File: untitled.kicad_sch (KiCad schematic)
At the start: 18 parts, among them J4 Pyro 2, J5 Pyro 1, Q1 FDS9926A, Q2 FDS4953, Q3 NDT3055L

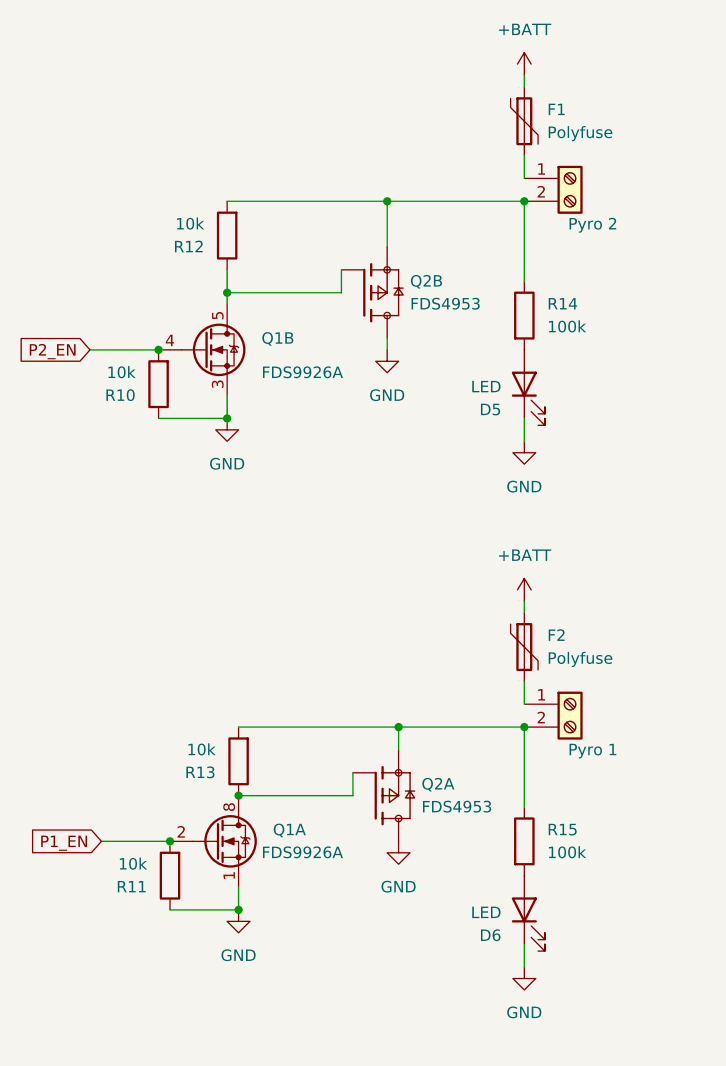
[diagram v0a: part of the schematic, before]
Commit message: V3
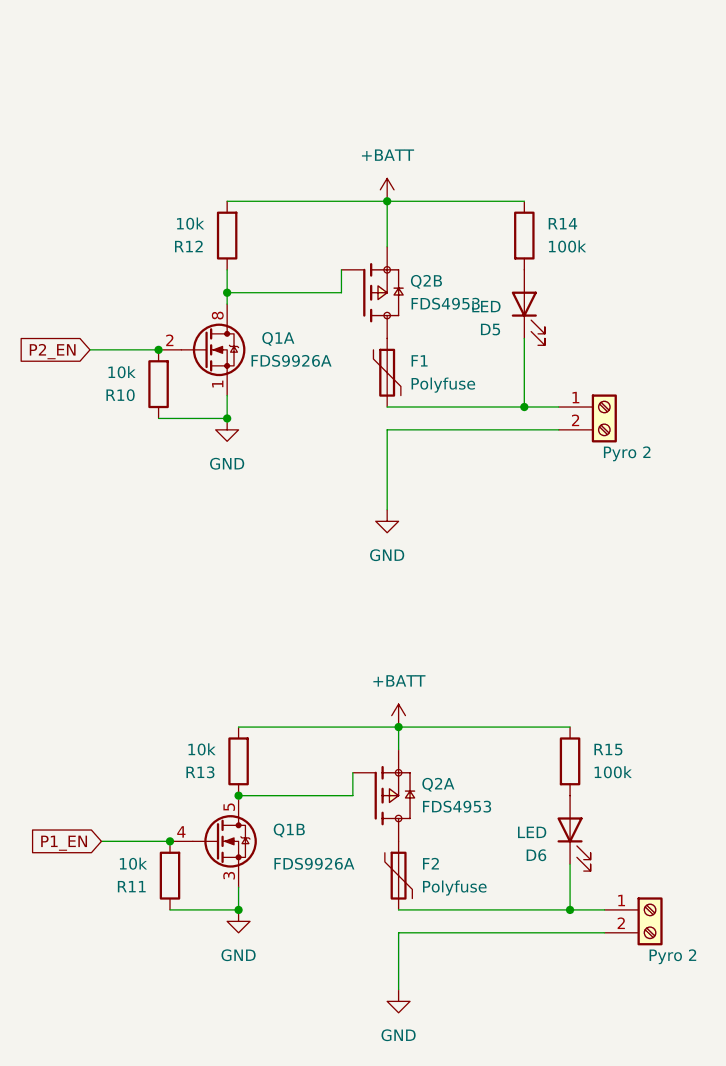
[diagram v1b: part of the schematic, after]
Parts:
- J4: footprint TerminalBlock_4Ucon:TerminalBlock_4Ucon_1x02_P3.50mm_Vertical -> TerminalBlock_Phoenix:TerminalBlock_Phoenix_MPT-0,5-2-2.54_1x02_P2.54mm_Horizontal
- J5: value Pyro 1 -> Pyro 2; footprint TerminalBlock_4Ucon:TerminalBlock_4Ucon_1x02_P3.50mm_Vertical -> TerminalBlock_Phoenix:TerminalBlock_Phoenix_MPT-0,5-2-2.54_1x02_P2.54mm_Horizontal
- Q3: footprint Package_TO_SOT_SMD:TSOT-23_HandSoldering -> Package_TO_SOT_SMD:TSOT-23
- R10, R11, R12, R13, R14, R15, R17, R18: footprint Resistor_SMD:R_0603_1608Metric_Pad0.98x0.95mm_HandSolder -> Resistor_SMD:R_0402_1005Metric_Pad0.72x0.64mm_HandSolder
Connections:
- net +BATT: now also Q2.1, Q2.3, R12.2, R13.2, R14.1, R15.1; no longer F1.1, F2.1
- net GND: now also J4.2 (Pin_2), J5.2 (Pin_2); no longer D5.1 (K), D6.1 (K), Q2.5, Q2.6, Q2.7, Q2.8
- net P1_EN: now also Q1.4 (G2); no longer Q1.2 (G1)
- net P2_EN: now also Q1.2 (G1); no longer Q1.4 (G2)
- net at F2.2, J5.1 (Pin_1): now also D6.1 (K)
- net at Q2.2, R12.1: now also Q1.7 (D1), Q1.8 (D1); no longer Q1.5 (D2), Q1.6 (D2)
- net at Q2.4, R13.1: now also Q1.5 (D2), Q1.6 (D2); no longer Q1.7 (D1), Q1.8 (D1)
- net at F1.2, J4.1 (Pin_1): now also D5.1 (K)
- new net: F2.1, Q2.5, Q2.6
- new net: F1.1, Q2.7, Q2.8
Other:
- moved on the sheet: D5, D6, F1, F2, Q1A, Q1B, R14, R15

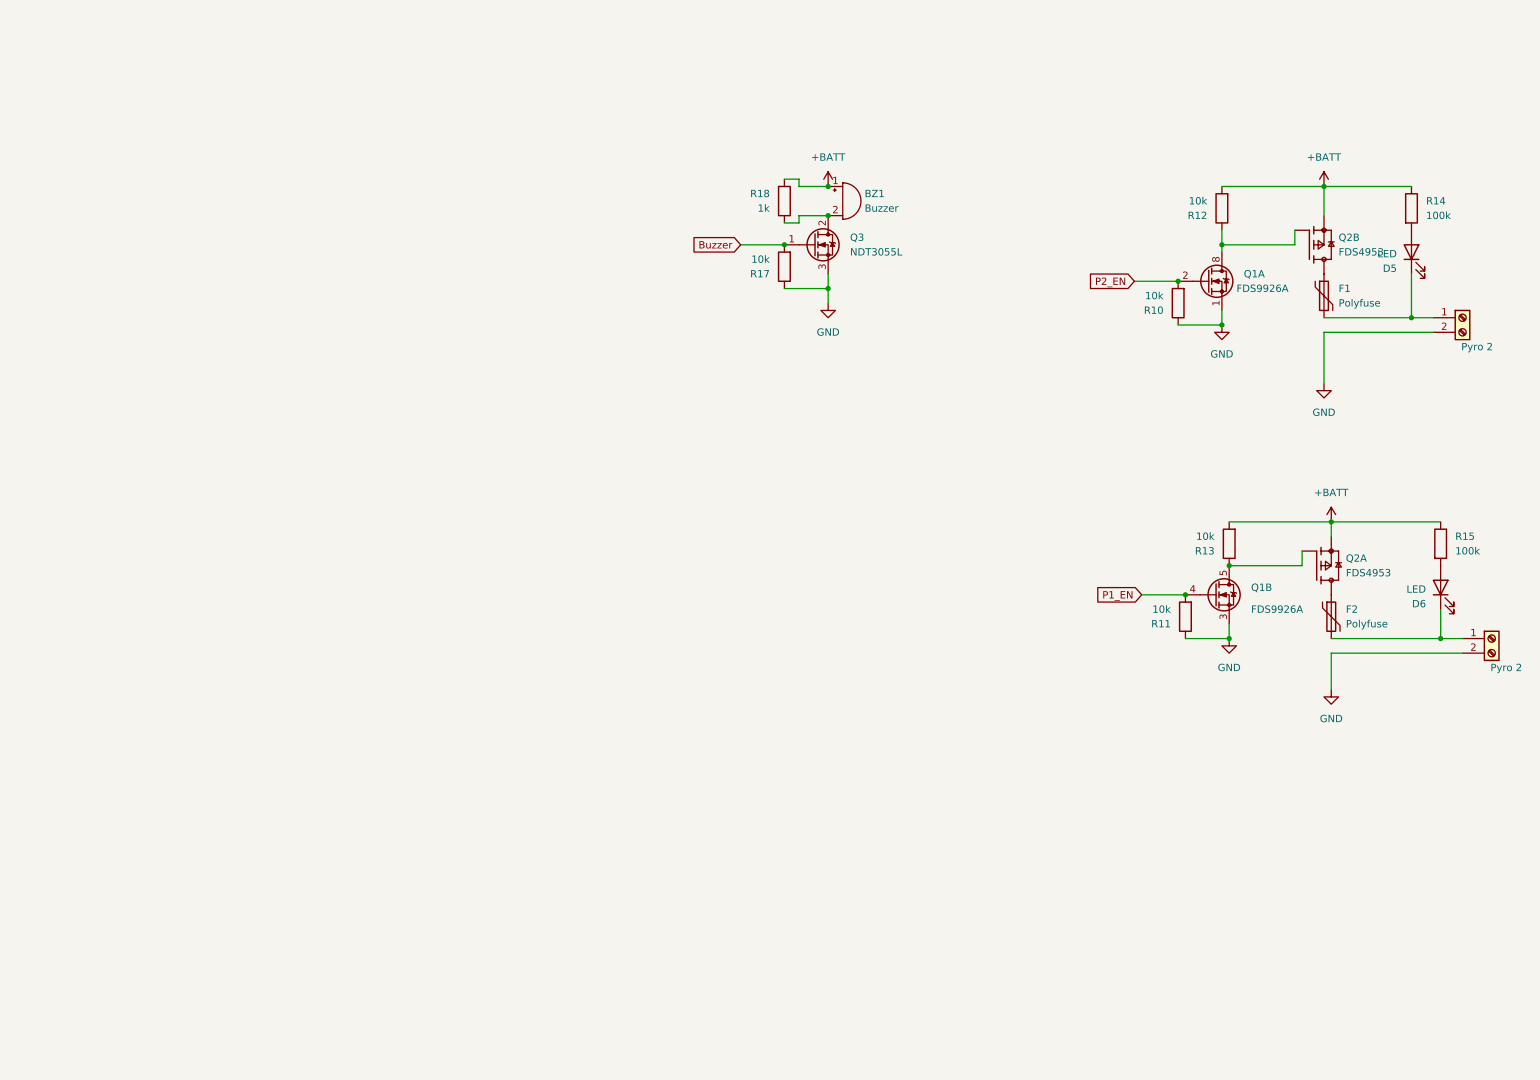
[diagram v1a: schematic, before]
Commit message: Rev 27052023
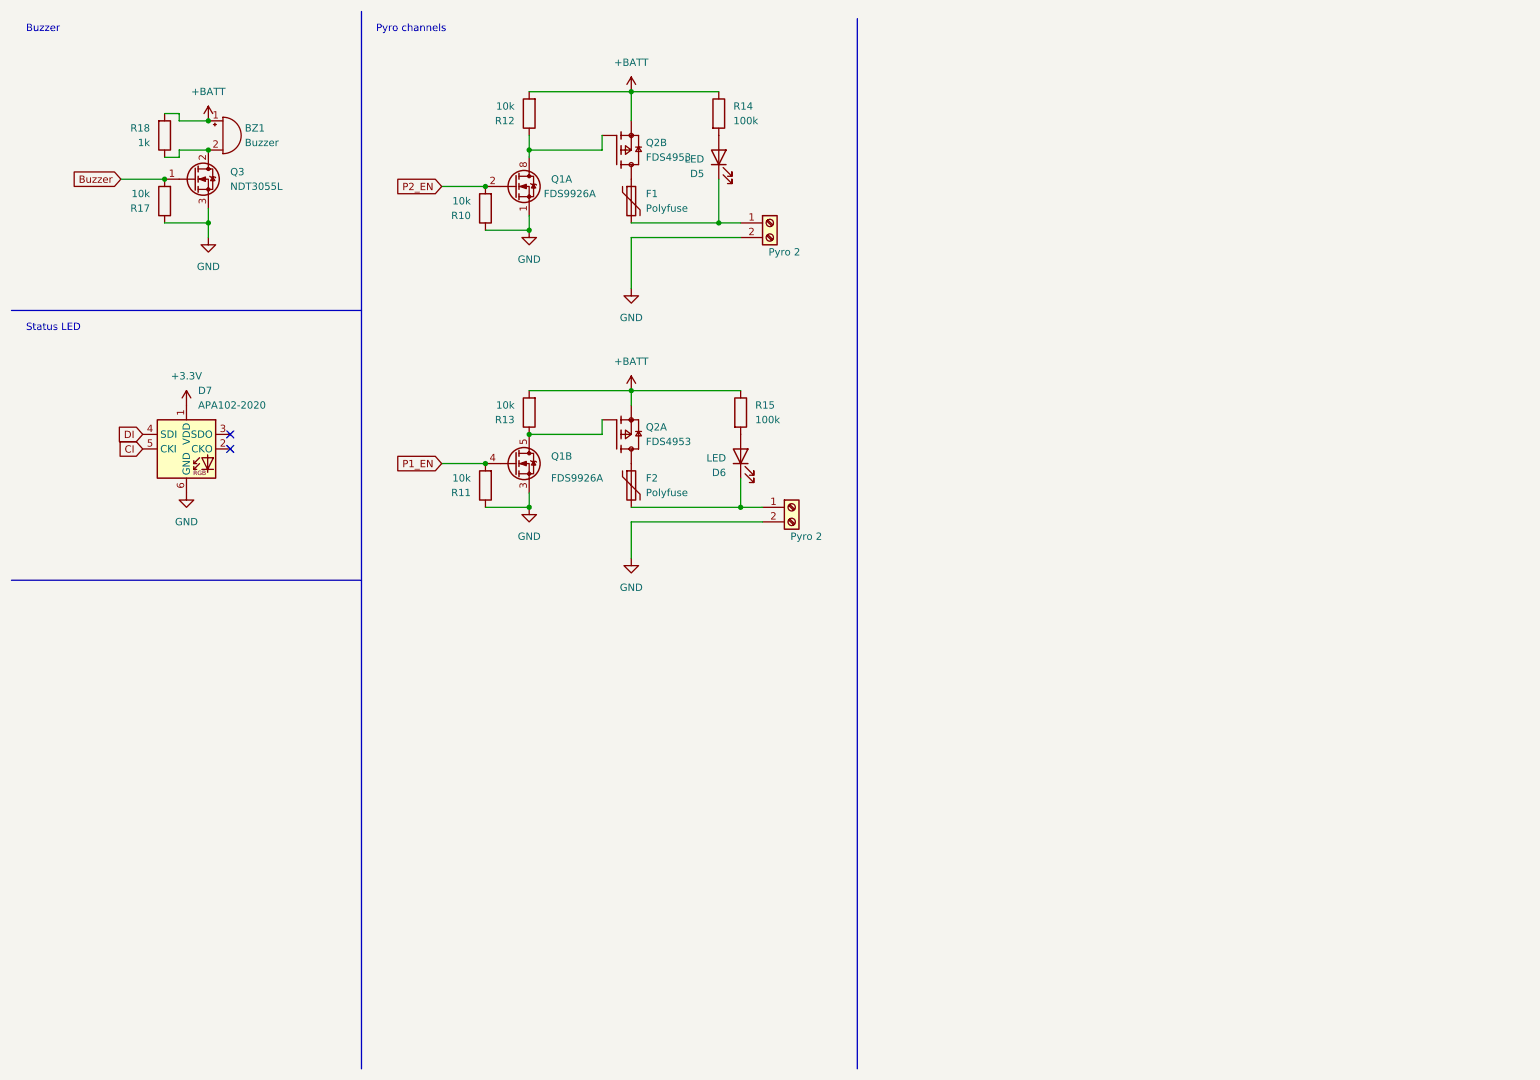
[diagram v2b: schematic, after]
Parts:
- added D7: APA102-2020, LED_SMD:LED-APA102-2020, symbol LED:APA102-2020
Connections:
- net GND: now also D7.6 (GND)
- new net +3V3: D7.1 (VDD)
- new net CI: D7.5 (CKI)
- new net DI: D7.4 (SDI)
- no-connect marks 0 -> 2
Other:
- note added: "Buzzer"
- note added: "Pyro channels"
- note added: "Status LED"
- moved on the sheet: BZ1, D5, D6, F1, F2, Q1A, Q1B, Q2A, Q2B, Q3, R10, R11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
